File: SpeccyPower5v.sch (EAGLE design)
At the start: 67 parts, among them T1 TRANS_ER29

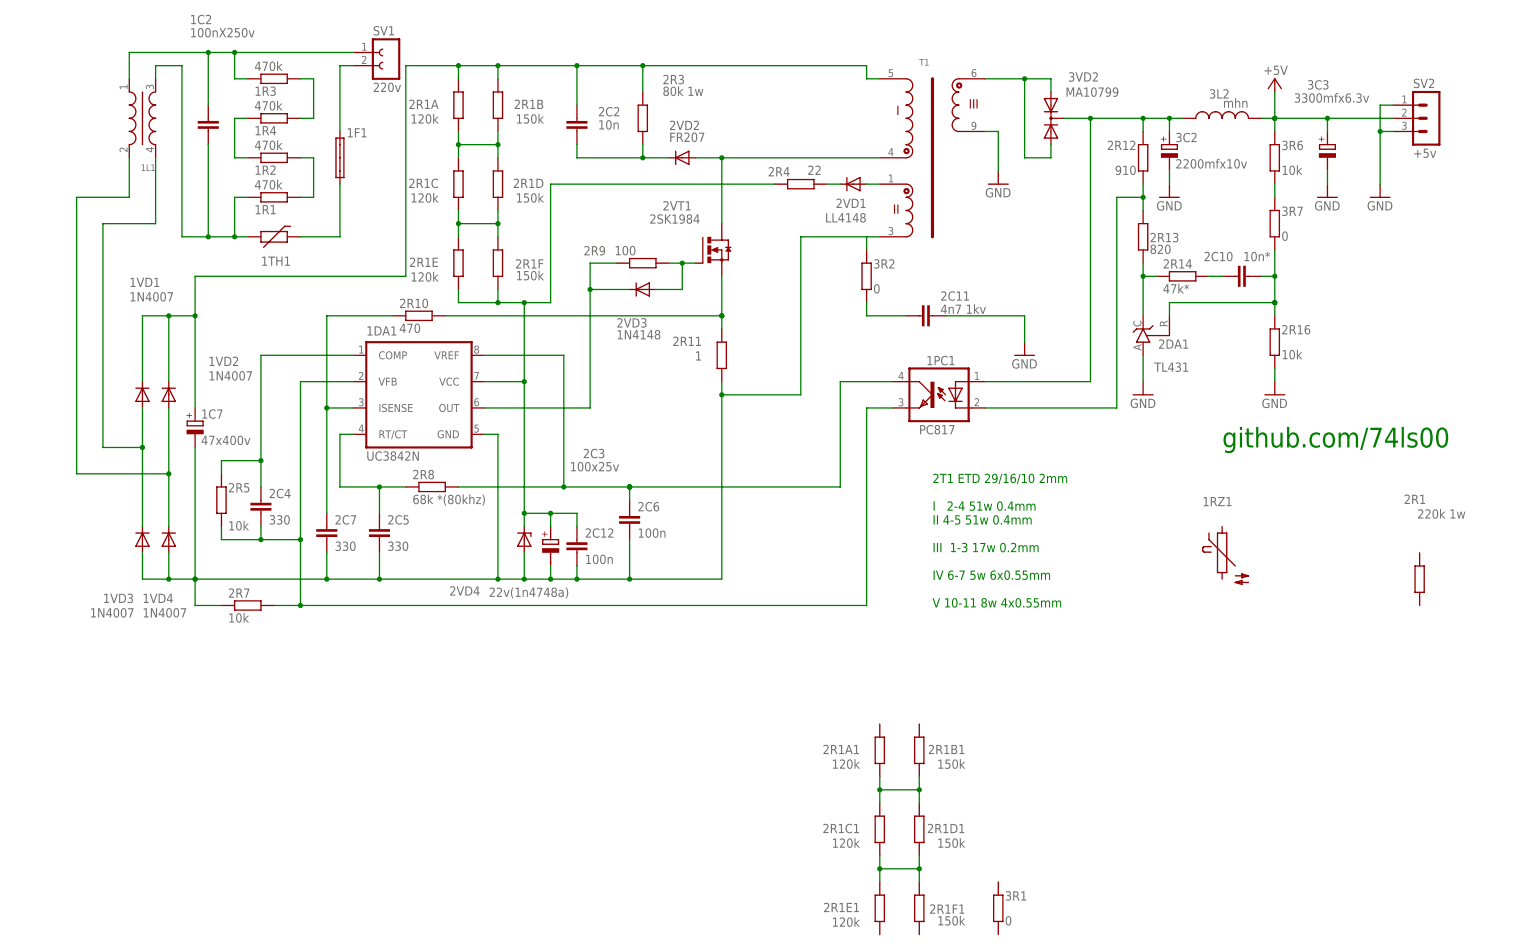
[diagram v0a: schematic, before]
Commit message: .
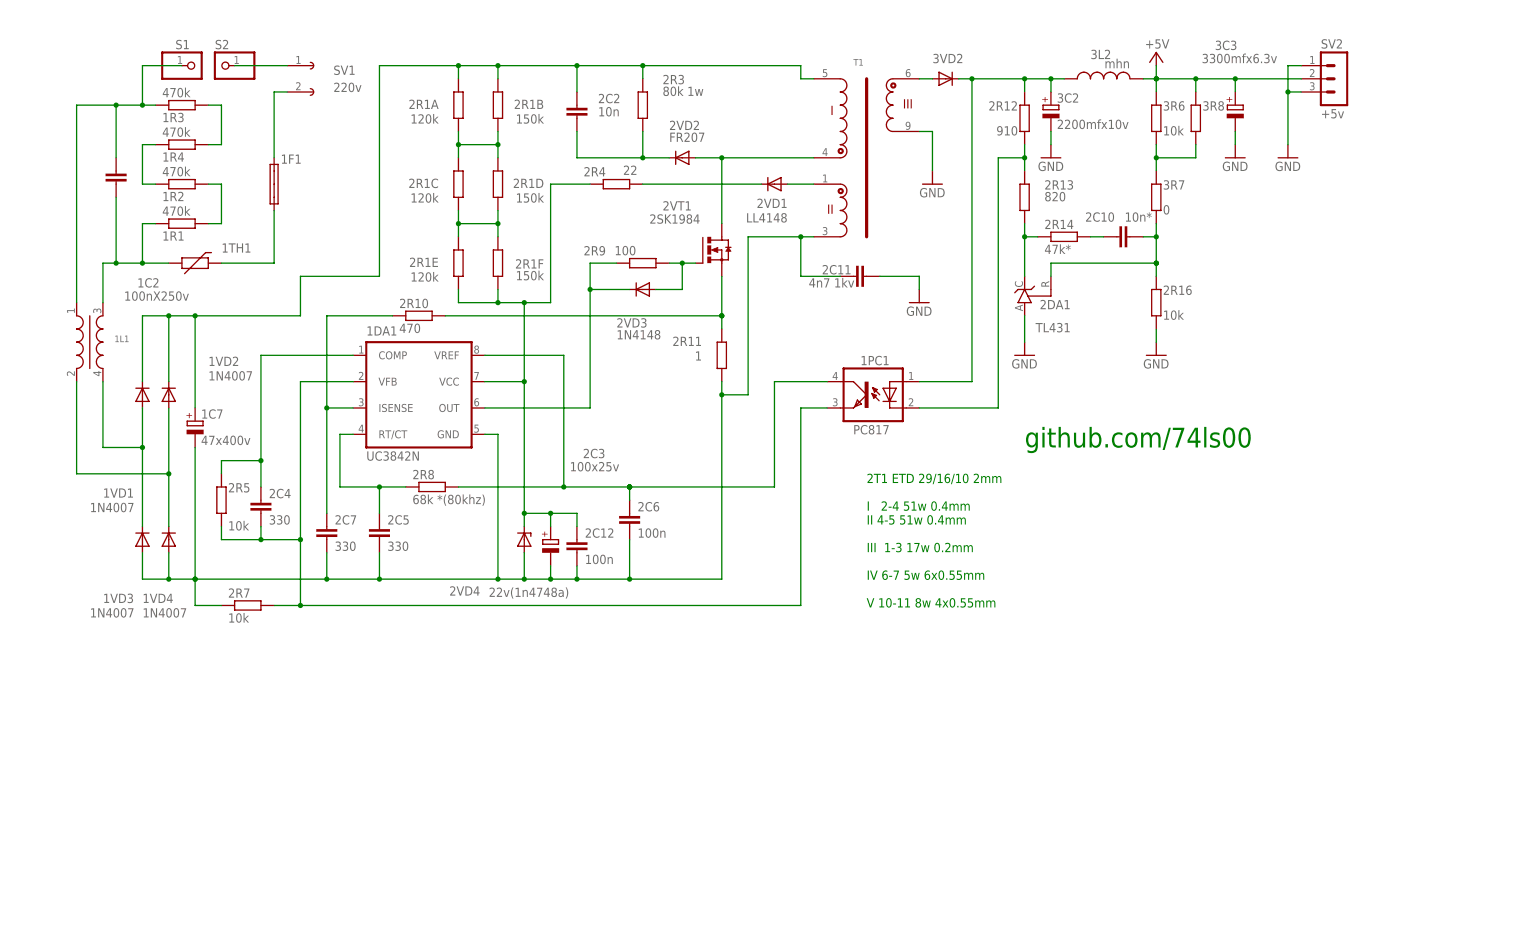
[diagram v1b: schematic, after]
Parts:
- removed 1RZ1: S1210, varistor:S1210
- removed 2R1: 220k 1w, rcl:R-EU_0613/15
- removed 2R1A1, 2R1C1, 2R1E1: 120k, rcl:R-EU_M0805
- removed 2R1B1, 2R1D1, 2R1F1: 150k, rcl:R-EU_M0805
- removed 3R1, 3R2: 0, rcl:R-EU_M1206
- added 3R8: (no value), rcl:R-EU_R0805
- added S1, S2: (no value), pinhead:PINHD-1X1
- 3VD2: value MA10799 -> (none); device diode:BYV32 -> diode:DIODE-DO220S
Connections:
- removed net N$27: 2R1C1.1, 2R1D1.1, 2R1E1.2, 2R1F1.1
- removed net N$31: 2R1A1.1, 2R1B1.1, 2R1C1.2, 2R1D1.2
- removed net N$33: 2C11.1, 3R2.1
- new net N$36: S2.1, SV1.1
- net +5V: now also 3R8.2
- net -IN: now also 2C11.1; no longer 3R2.2
- net N$26: now also 3R8.1
- net N$28: now also 3VD2.A; no longer 3VD2.A1, 3VD2.A2
- net N$32: now also S1.1; no longer SV1.1
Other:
- moved on the sheet: 1C2, 1F1, 1L1, 1PC1, 1R1, 1R2, 1R3, 1R4, 1TH1, 2C10, 2C11, 2C2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

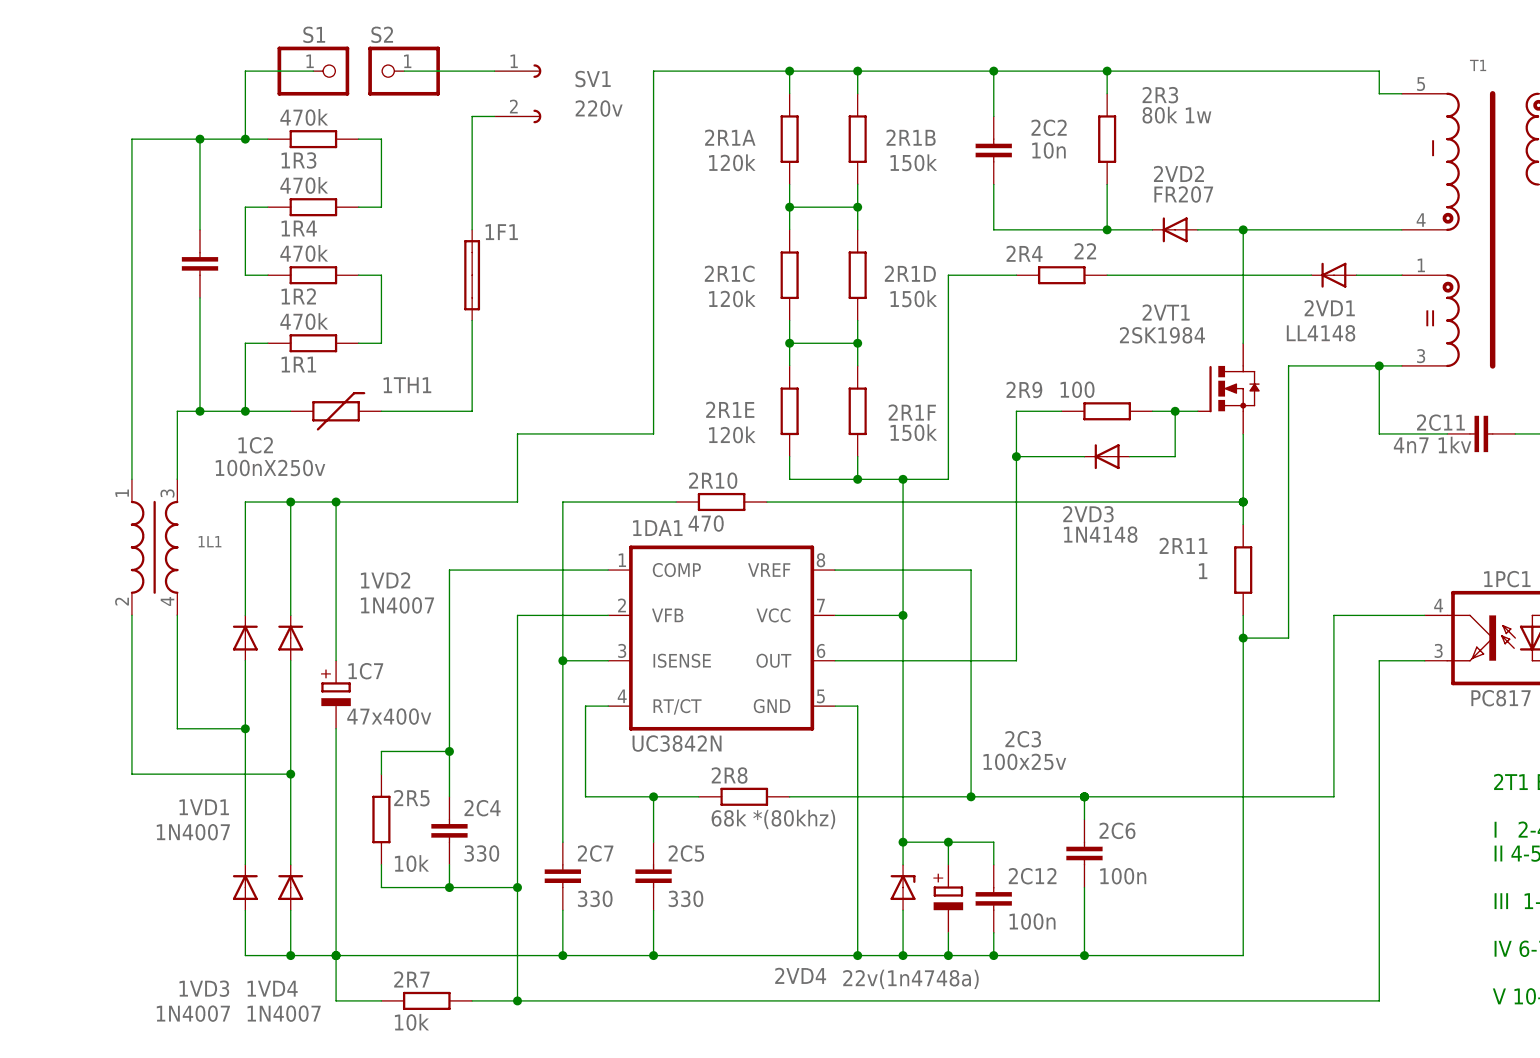
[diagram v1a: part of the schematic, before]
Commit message: test v h
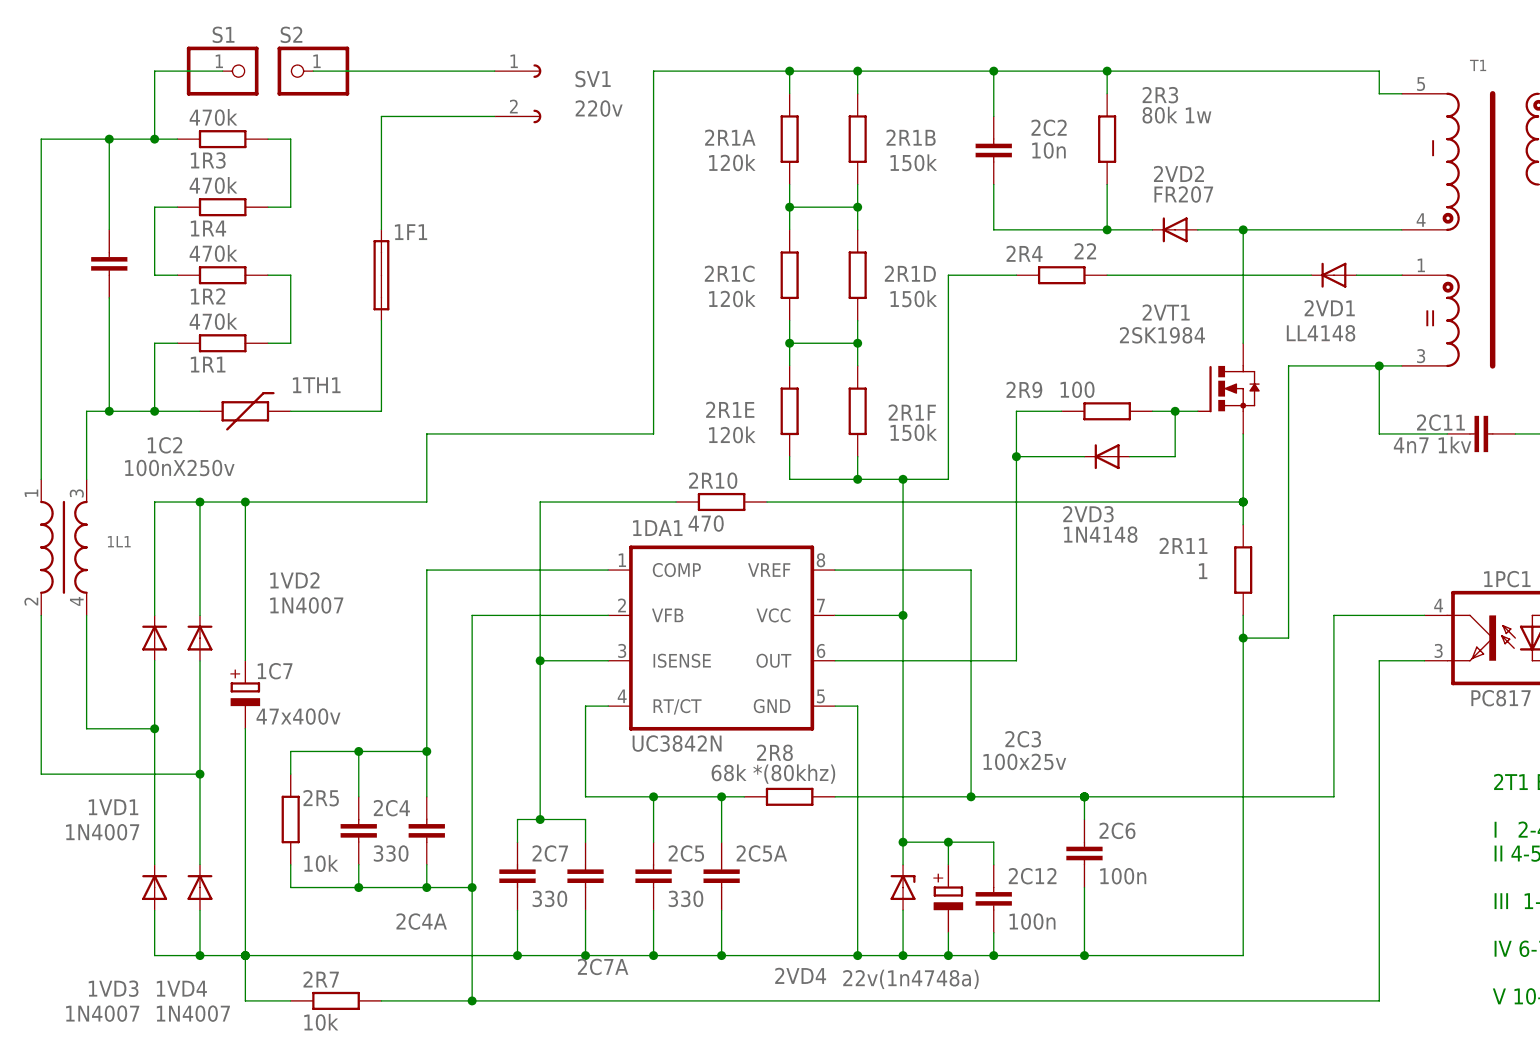
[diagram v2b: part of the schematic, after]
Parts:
- added 2C4A, 2C5A, 2C7A: (no value), rcl:C-EUC0805
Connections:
- net N$23 renamed +IN
- removed net N$40: 1DA1.VFB, 1PC1.EMIT, 2C4.2, 2R5.1, 2R7.2
- removed net N$6: 1DA1.COMP, 2C4.1, 2R5.2
- new net 817-3: 1DA1.VFB, 1PC1.EMIT, 2C4.2, 2C4A.2, 2R5.1, 2R7.2
- new net COMP: 1DA1.COMP, 2C4.1, 2C4A.1, 2R5.2
- net -IN: now also 2C5A.2, 2C7A.2
- net N$3: now also 2C5A.1
- net N$4: now also 2C7A.1
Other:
- moved on the sheet: 1C2, 1C7, 1F1, 1L1, 1R1, 1R2, 1R3, 1R4, 1TH1, 1VD1, 1VD2, 1VD3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

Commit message: ..
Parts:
- 2R13: device rcl:R-EU_0207/10 -> rcl:R-EU_0204/7
- 2VD2: device SpeccyPower5v:1N4148DO35-10 -> SpeccyPower5v:1N4148DO35-7
- 3L2: device rcl:L-USTFI0305 -> rcl:L-USLAL02
- 3R7: device rcl:R-EU_M1206 -> rcl:R-EU_M0805
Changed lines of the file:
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@@
 <part name="2VD3" library="SpeccyPower5v" deviceset="1N4148" device="DO35-7" value="1N4148"/>
 <part name="2R12" library="rcl" deviceset="R-EU_" device="R0805" value="910"/>
-<part name="2R13" library="rcl" deviceset="R-EU_" device="0207/10" value="820"/>
+<part name="2R13" library="rcl" deviceset="R-EU_" device="0204/7" value="820"/>
 <part name="2DA1" library="v-reg" deviceset="TL431CLP" device="" value="TL431"/>
 <part name="2R14" library="rcl" deviceset="R-EU_" device="R0805" value="47k*"/>
@@
 <part name="1F1" library="fuse" deviceset="SHK20L" device=""/>
 <part name="GND5" library="supply1" deviceset="GND" device=""/>
-<part name="2VD2" library="SpeccyPower5v" deviceset="1N4148" device="DO35-10" value="FR207"/>
+<part name="2VD2" library="SpeccyPower5v" deviceset="1N4148" device="DO35-7" value="FR207"/>
 <part name="1VD1" library="diode" deviceset="1N4004" device="" value="1N4007"/>
 <part name="1VD2" library="diode" deviceset="1N4004" device="" value="1N4007"/>
@@
 <part name="3C2" library="SpeccyPower5v" deviceset="CPOL-EU" device="TT2D7L" value="2200mfx10v"/>
 <part name="3C3" library="SpeccyPower5v" deviceset="CPOL-EU" device="TT2D7L" value="3300mfx6.3v"/>
-<part name="3L2" library="rcl" deviceset="L-US" device="TFI0305" value="mhn"/>
+<part name="3L2" library="rcl" deviceset="L-US" device="LAL02" value="mhn"/>
 <part name="GND9" library="supply1" deviceset="GND" device=""/>
 <part name="GND10" library="supply1" deviceset="GND" device=""/>
@@
 <part name="SV2" library="con-lstb" deviceset="MA03-1" device="" value="+5v"/>
 <part name="GND1" library="supply1" deviceset="GND" device=""/>
-<part name="3R7" library="rcl" deviceset="R-EU_" device="M1206" value="0"/>
+<part name="3R7" library="rcl" deviceset="R-EU_" device="M0805" value="0"/>
 <part name="3VD2" library="diode" deviceset="DIODE-" device="DO220S"/>
 <part name="3R8" library="rcl" deviceset="R-EU_" device="R0805"/>

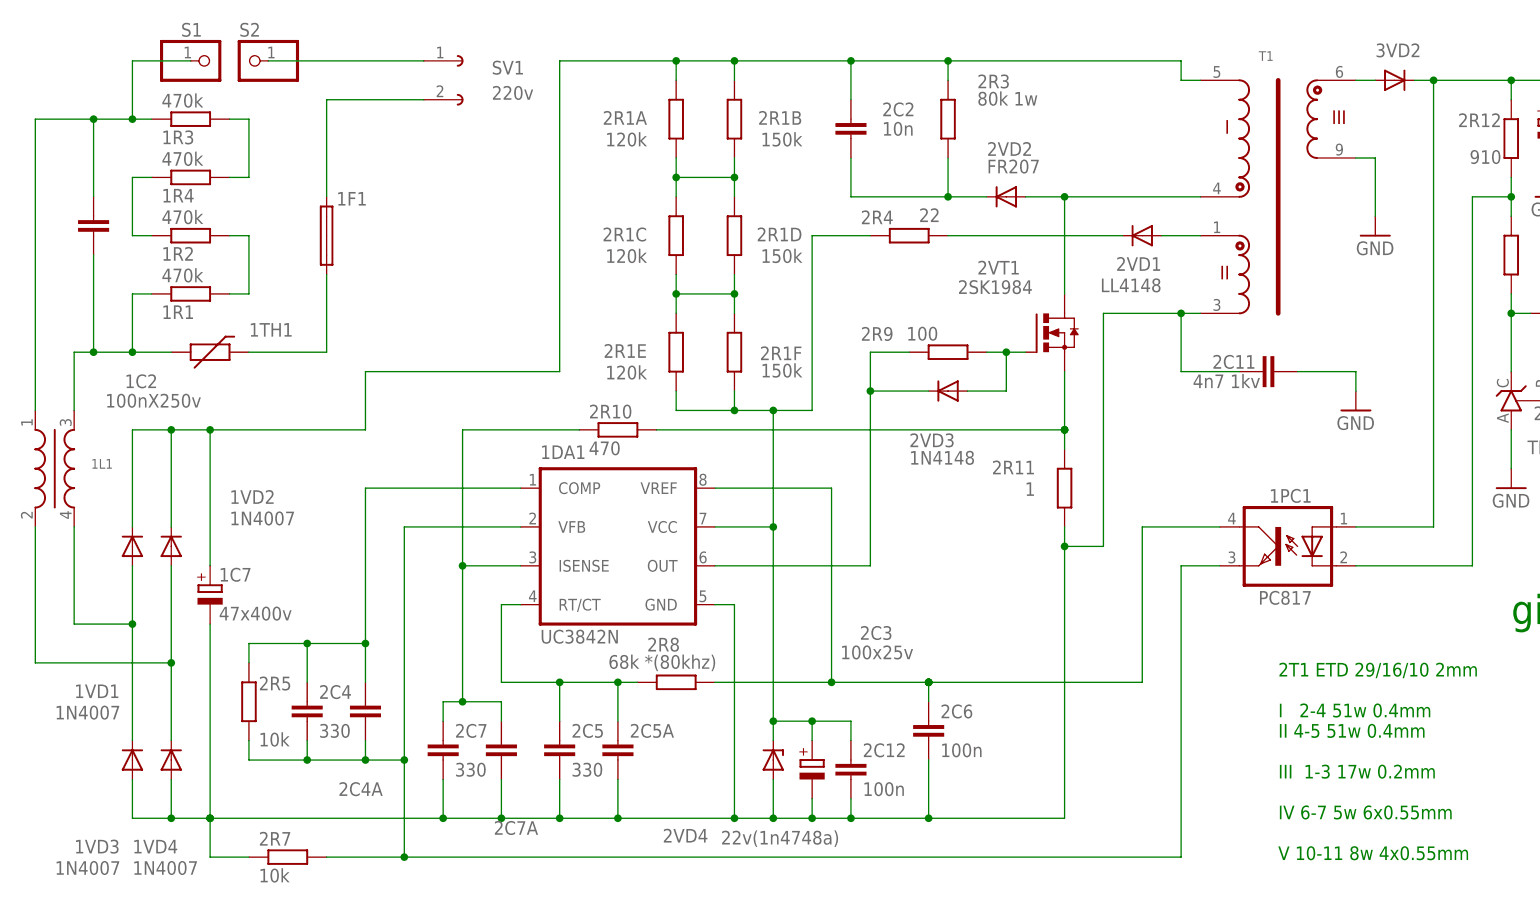
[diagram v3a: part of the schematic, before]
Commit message: ..
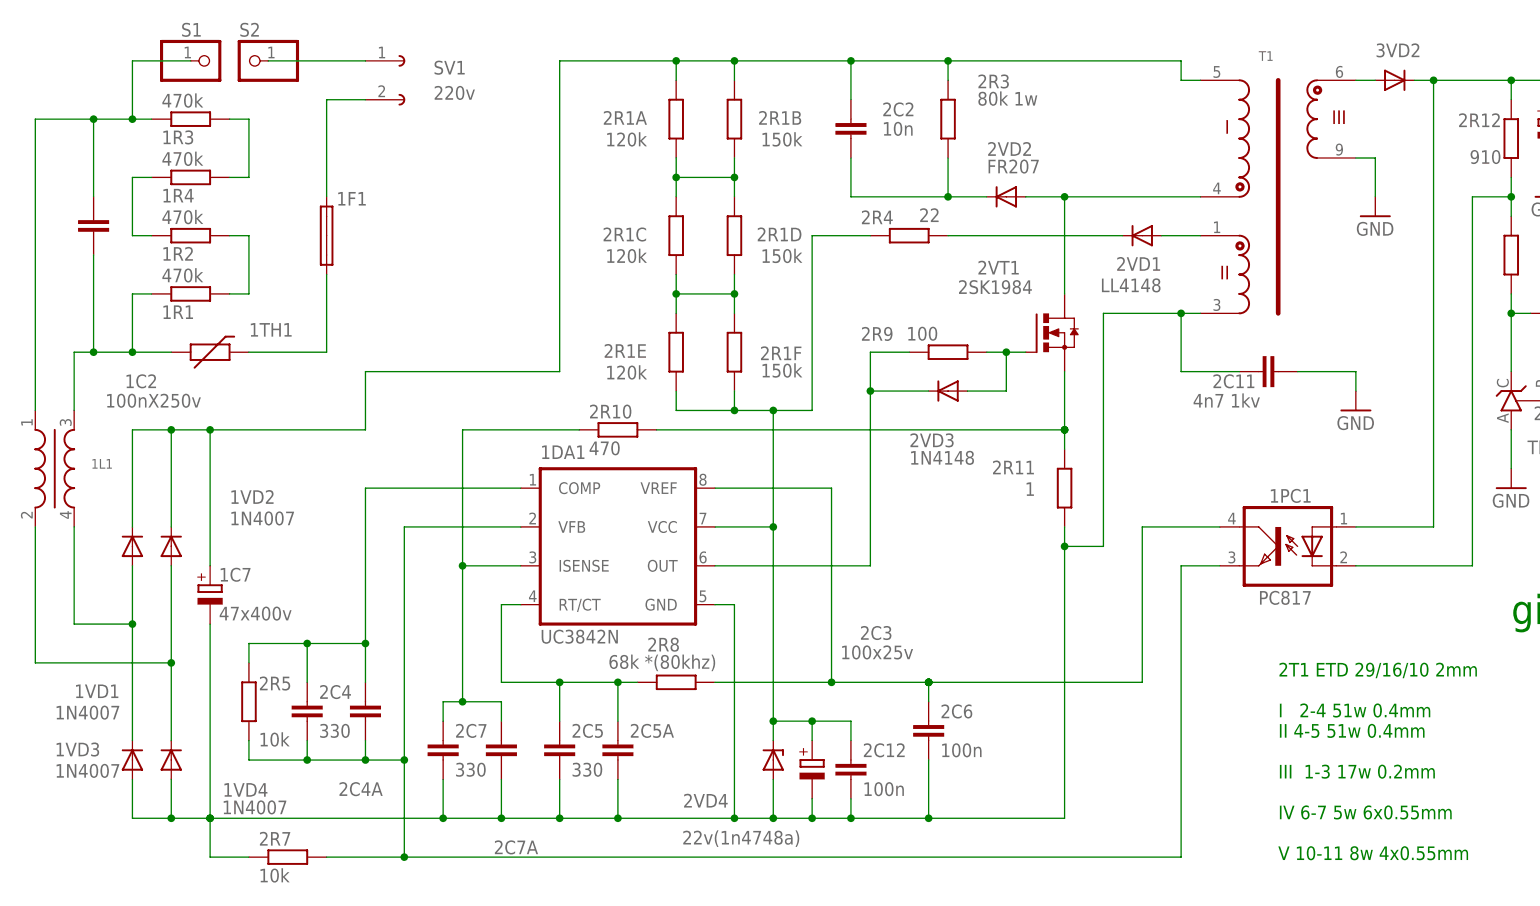
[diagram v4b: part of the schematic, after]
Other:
- moved on the sheet: SV1
